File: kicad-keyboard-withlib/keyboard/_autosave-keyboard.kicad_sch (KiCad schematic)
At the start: 45 parts, among them SW1 SW_Push, SW10 SW_Push, SW11 SW_Push, SW12 SW_Push, SW13 SW_Push, SW14 SW_Push, SW15 SW_Push, SW16 SW_Push, SW17 SW_Push, SW18 SW_Push, SW19 SW_Push, SW2 SW_Push, SW20 SW_Push, SW21 SW_Push, SW22 SW_Push, SW23 SW_Push, SW24 SW_Push, SW25 SW_Push, SW26 SW_Push, SW27 SW_Push, SW28 SW_Push, SW29 SW_Push, SW3 SW_Push, SW30 SW_Push, SW31 SW_Push, SW32 SW_Push, SW33 SW_Push, SW34 SW_Push, SW35 SW_Push, SW36 SW_Push, SW37 SW_Push, SW38 SW_Push, SW39 SW_Slide_DPDT, SW4 SW_Push, SW41 RotaryEncoder_Switch, SW5 SW_Push, SW6 SW_Push, SW7 SW_Push, SW8 SW_Push, SW9 SW_Push, U2 MCP23017_SO

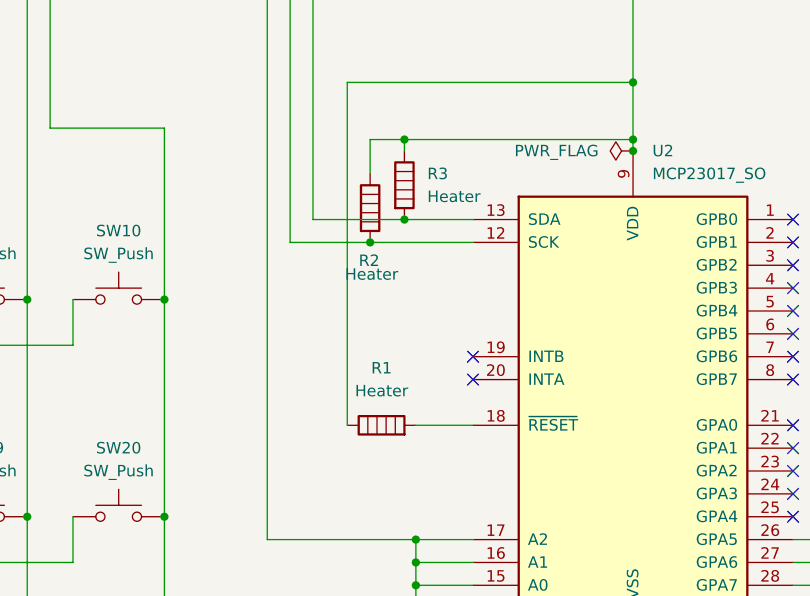
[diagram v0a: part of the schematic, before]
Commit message: fix post Christian
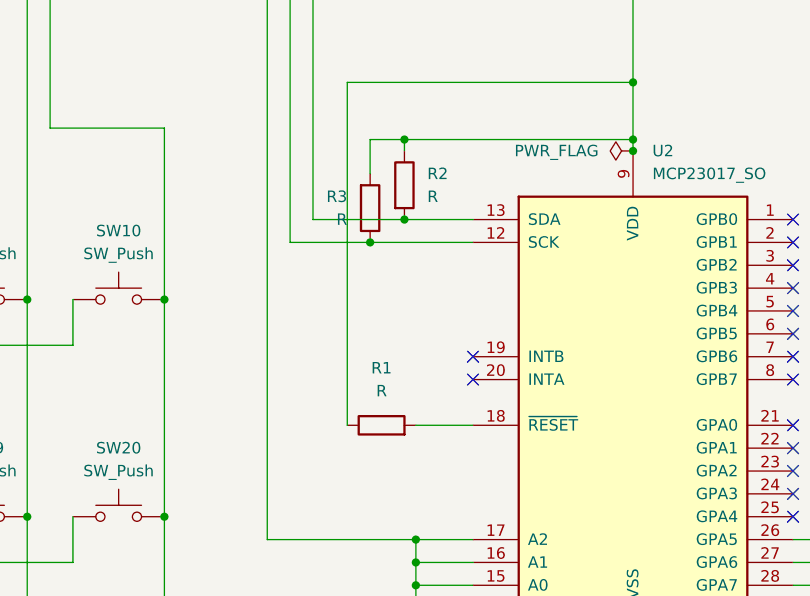
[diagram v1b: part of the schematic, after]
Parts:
- removed R1, R2, R3: Heater, Resistor_SMD:R_0201_0603Metric, symbol Device:Heater
- added R1, R2, R3: R, Resistor_SMD:R_0603_1608Metric_Pad0.98x0.95mm_HandSolder, symbol Device:R
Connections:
- net at P1.16 (VCC), U2.9 (VDD): now also R1.1, R2.1, R3.2
- net at P1.21 (SCL), U2.12 (SCK): now also R3.1
- net at P1.20 (SDA), U2.13 (SDA): now also R2.2
- net at U2.18 (~{RESET}): now also R1.2
